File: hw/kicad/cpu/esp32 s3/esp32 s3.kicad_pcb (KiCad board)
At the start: 2 copper layers, 40 x 40 mm, 18 parts, among them J1 TOP, J2 BUTTOM, J3 USB_B_Micro, SW1 SW_Push, SW2 SW_Push, U1 ESP32-S3-WROOM-1-N16R2, U2 ICM-42688-P

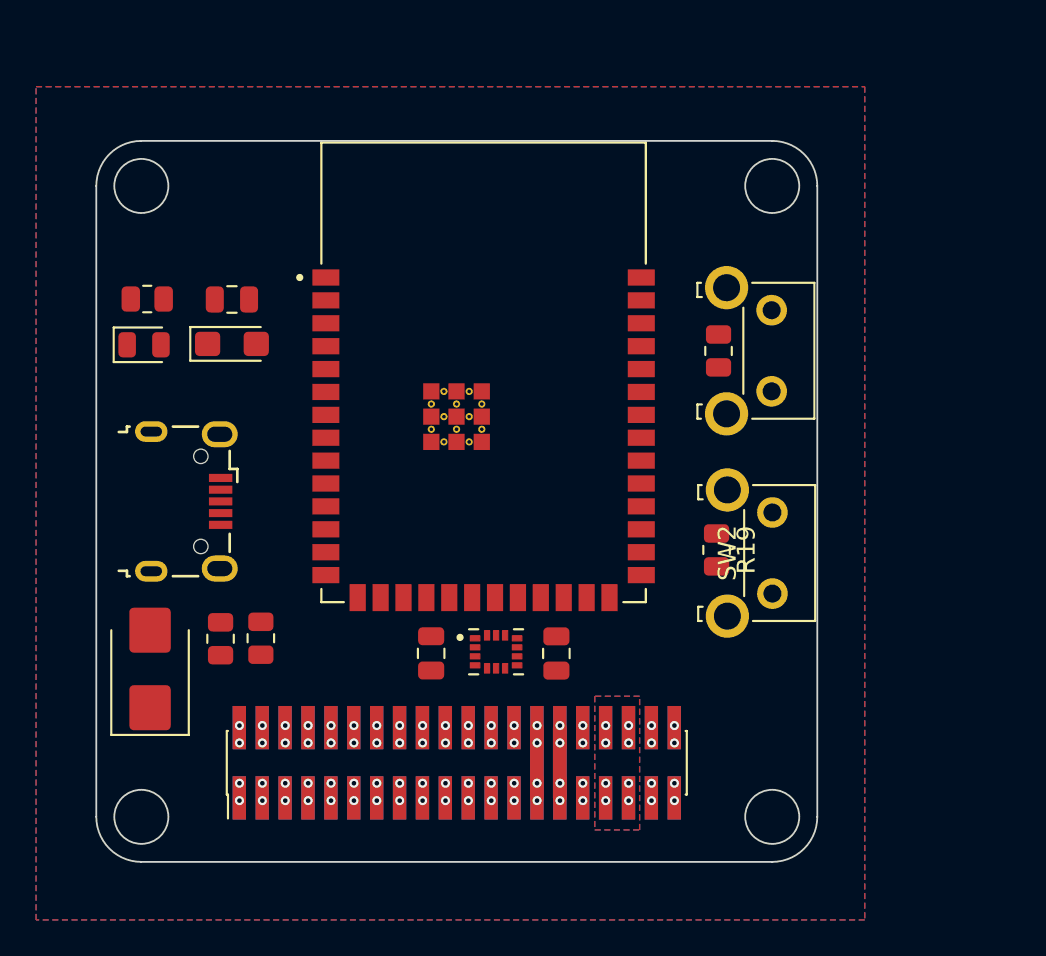
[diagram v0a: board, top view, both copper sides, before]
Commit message: Merge from normal
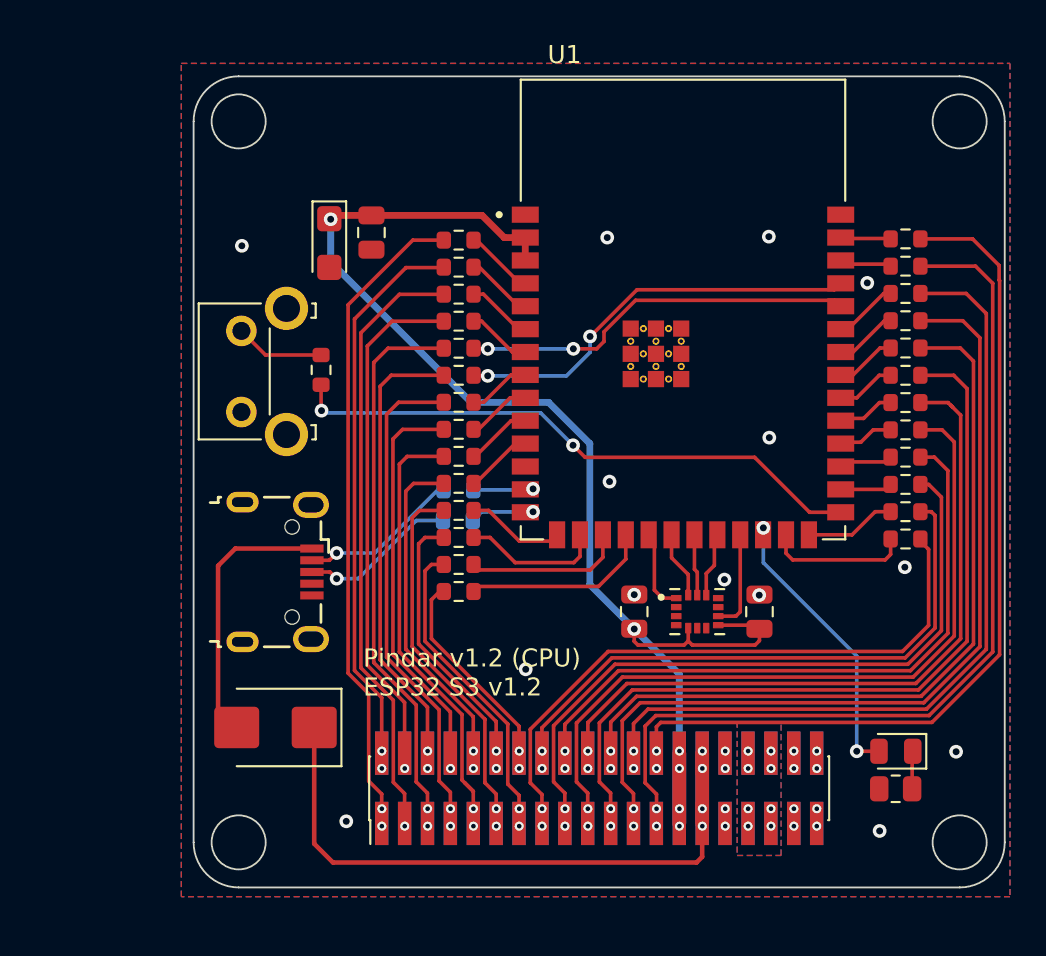
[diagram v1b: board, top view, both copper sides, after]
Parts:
- removed SW2: SW_Push, Button_Switch_THT:SW_SPST_Omron_B3F-315x_Angled
- added R10: R, Resistor_SMD:R_0603_1608Metric, F.Cu at (65.4, 52.3)
- added R11: R, Resistor_SMD:R_0603_1608Metric, F.Cu at (65.4, 53.8)
- added R12: R, Resistor_SMD:R_0603_1608Metric, F.Cu at (65.4, 55.3)
- added R13: R, Resistor_SMD:R_0603_1608Metric, F.Cu at (65.4, 56.8)
- added R14: R, Resistor_SMD:R_0603_1608Metric, F.Cu at (65.4, 58.3)
- added R15: R, Resistor_SMD:R_0603_1608Metric, F.Cu at (65.4, 59.8)
- added R16: R, Resistor_SMD:R_0603_1608Metric, F.Cu at (65.4, 61.3)
- added R17: R, Resistor_SMD:R_0603_1608Metric, F.Cu at (90.2, 58.4)
- added R18: R, Resistor_SMD:R_0603_1608Metric, F.Cu at (90.2, 56.9)
- added R20: R, Resistor_SMD:R_0603_1608Metric, F.Cu at (90.2, 53.8)
- added R21: R, Resistor_SMD:R_0603_1608Metric, F.Cu at (90.2, 52.3)
- added R22: R, Resistor_SMD:R_0603_1608Metric, F.Cu at (90.2, 50.8)
- added R23: R, Resistor_SMD:R_0603_1608Metric, F.Cu at (90.2, 49.3)
- added R24: R, Resistor_SMD:R_0603_1608Metric, F.Cu at (90.2, 47.8)
- added R25: R, Resistor_SMD:R_0603_1608Metric, F.Cu at (90.2, 46.3)
- added R26: R, Resistor_SMD:R_0603_1608Metric, F.Cu at (90.2, 44.8)
- added R27: R, Resistor_SMD:R_0603_1608Metric, F.Cu at (90.2, 43.3)
- added R28: R, Resistor_SMD:R_0603_1608Metric, F.Cu at (90.2, 41.7)
- added R3: R, Resistor_SMD:R_0603_1608Metric, F.Cu at (65.4, 41.8)
- added R4: R, Resistor_SMD:R_0603_1608Metric, F.Cu at (65.4, 43.3)
- added R5: R, Resistor_SMD:R_0603_1608Metric, F.Cu at (65.4, 44.8)
- added R6: R, Resistor_SMD:R_0603_1608Metric, F.Cu at (65.4, 46.3)
- added R7: R, Resistor_SMD:R_0603_1608Metric, F.Cu at (65.4, 47.8)
- added R8: R, Resistor_SMD:R_0603_1608Metric, F.Cu at (65.4, 49.3)
- added R9: R, Resistor_SMD:R_0603_1608Metric, F.Cu at (65.4, 50.8)
- R1: footprint Resistor_SMD:R_0805_2012Metric -> Resistor_SMD:R_0603_1608Metric
- R19: value 1k -> R; footprint Resistor_SMD:R_0805_2012Metric -> Resistor_SMD:R_0603_1608Metric
- R29, R30: footprint Resistor_SMD:R_0805_2012Metric -> Resistor_SMD:R_0603_1608Metric; moved to B.Cu
- moved R2 49.6 mm to (89.7, 72.2)
- moved D1 47.4 mm to (89.7, 70.2), turned to 180 degrees
- moved SW1 30.0 mm to (53.4, 51.3), turned to 90 degrees
- moved R1 22.1 mm to (57.8, 49.0)
- moved R30 15.6 mm to (65.4, 55.7), turned to 0 degrees
- moved R29 12.7 mm to (65.4, 57.4), turned to 0 degrees
- moved U1 11.6 mm to (77.9, 45.7)
- moved C3 11.5 mm to (75.2, 62.4)
- moved C4 11.5 mm to (82.1, 62.4)
- moved U2 11.4 mm to (78.7, 62.4)
- moved R19 11.1 mm to (90.2, 55.4), turned to 0 degrees
- moved C2 8.58 mm to (60.6, 41.4), turned to -90 degrees
- moved J1 8.02 mm to (73.2, 72.2)
- moved J2 8.02 mm to (73.2, 72.2)
- moved C1 7.78 mm to (58.2, 42.0), turned to -90 degrees
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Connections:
- R1 pad 1: GND -> Net-(R1-Pad1)
- R1 pad 2: Net-(R1-Pad2) -> Net-(U1-IO0)
- R19 pad 1: GND -> /gpio3
- R19 pad 2: Net-(R19-Pad2) -> /GPIO_3
- SW1 pad 1: Net-(R1-Pad2) -> GND
- SW1 pad 2: Net-(U1-IO0) -> Net-(R1-Pad1)
- U1 pad 10: /I2C_SDA -> /i2c_sda
- U1 pad 11: /I2C_CLK -> /i2c_clk
- U1 pad 12: /LED -> unconnected-(U1-IO8-Pad12)
- U1 pad 15: /SPI_MISO -> /spi3_cs
- U1 pad 16: /SPI_CS -> /spi3_clk
- U1 pad 17: /SPI_MOSI -> /spi3_mosi
- U1 pad 18: /SPI_CLK -> /spi3_miso
- U1 pad 19: /spi3_miso -> /spi2_miso
- U1 pad 20: /IMU_FSYNC -> /spi2_mosi
- U1 pad 21: /spi3_cs -> /spi2_clk
- U1 pad 22: /spi3_clk -> /spi2_cs
- U1 pad 23: /spi3_mosi -> /IMU_FSYNC
- U1 pad 24: /GPIO_1 -> /LED
- U1 pad 25: /GPIO_2 -> /gpio1
- U1 pad 26: Net-(U1-IO45) -> /gpio2
- U1 pad 28: /GPIO_3 -> /gpio3
- U1 pad 29: /GPIO_4 -> /gpio4
- U1 pad 30: /GPIO_5 -> /gpio5
- U1 pad 31: /GPIO_6 -> /gpio6
- U1 pad 32: /GPIO_7 -> /gpio7
- U1 pad 33: /GPIO_8 -> /gpio8
- U1 pad 34: /GPIO_9 -> /gpio9
- U1 pad 35: /GPIO_10 -> /gpio10
- U1 pad 36: /UART1_Rx -> /uart0_rx
- U1 pad 37: /UART1_Tx -> /uart0_tx
- U1 pad 38: /GPIO_11 -> /gpio11
- U1 pad 39: /GPIO_12 -> /gpio12
- U1 pad 4: /ADC_1 -> /adc1_ch3
- U1 pad 41_10: (no net) -> GND
- U1 pad 41_11: (no net) -> GND
- U1 pad 41_12: (no net) -> GND
- U1 pad 41_13: (no net) -> GND
- U1 pad 41_14: (no net) -> GND
- U1 pad 41_15: (no net) -> GND
- U1 pad 41_16: (no net) -> GND
- U1 pad 41_17: (no net) -> GND
- U1 pad 41_18: (no net) -> GND
- U1 pad 41_19: (no net) -> GND
- U1 pad 41_20: (no net) -> GND
- U1 pad 41_21: (no net) -> GND
- U1 pad 5: /ADC_2 -> /adc1_ch4
- U1 pad 6: /ADC_3 -> /adc1_ch5
- U1 pad 7: /ADC_4 -> /adc1_ch6
- U1 pad 8: /UART2_Rx -> /uart1_rx
- U1 pad 9: /UART2_Tx -> /uart1_tx
- U2 pad 1: /spi3_miso -> /spi2_miso
- U2 pad 12: /spi3_cs -> /spi2_cs
- U2 pad 13: /spi3_clk -> /spi2_clk
- U2 pad 14: /spi3_mosi -> /spi2_mosi
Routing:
- net +3.3V: track 7.80 -> 72.4 mm, vias 4 -> 6
- net /GPIO_11: track 0.00 -> 50.7 mm
- net /GPIO_12: track 0.00 -> 48.7 mm
- net /GPIO_9: track 0.00 -> 48.3 mm
- net /GPIO_10: track 0.00 -> 45.7 mm
- net /GPIO_7: track 0.00 -> 45.0 mm
- net /GPIO_8: track 0.00 -> 42.5 mm
- net /GPIO_5: track 0.00 -> 41.7 mm
- net /GPIO_6: track 0.00 -> 39.3 mm
- net /GPIO_3: track 0.00 -> 38.3 mm
- net /ADC_1: track 0.00 -> 36.3 mm
- net /GPIO_4: track 0.00 -> 35.8 mm
- net /GPIO_1: track 0.00 -> 35.0 mm
- net /ADC_3: track 0.00 -> 33.7 mm, vias 2 -> 1
- net /GPIO_2: track 0.00 -> 32.7 mm
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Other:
- board size 40 x 40 mm -> 45 x 45 mm
- board text added: "Pindar v1.2 (CPU) ESP32 S3 v1.2"
